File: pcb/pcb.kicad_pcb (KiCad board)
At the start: 2 copper layers, 7 parts, among them J1 Conn_01x16_Socket, J2 USB_C_Receptacle, U1 W65C02SxP, U2 W65C22SxP, U3 28C256, U4 28C256, U5 HM62256BLP

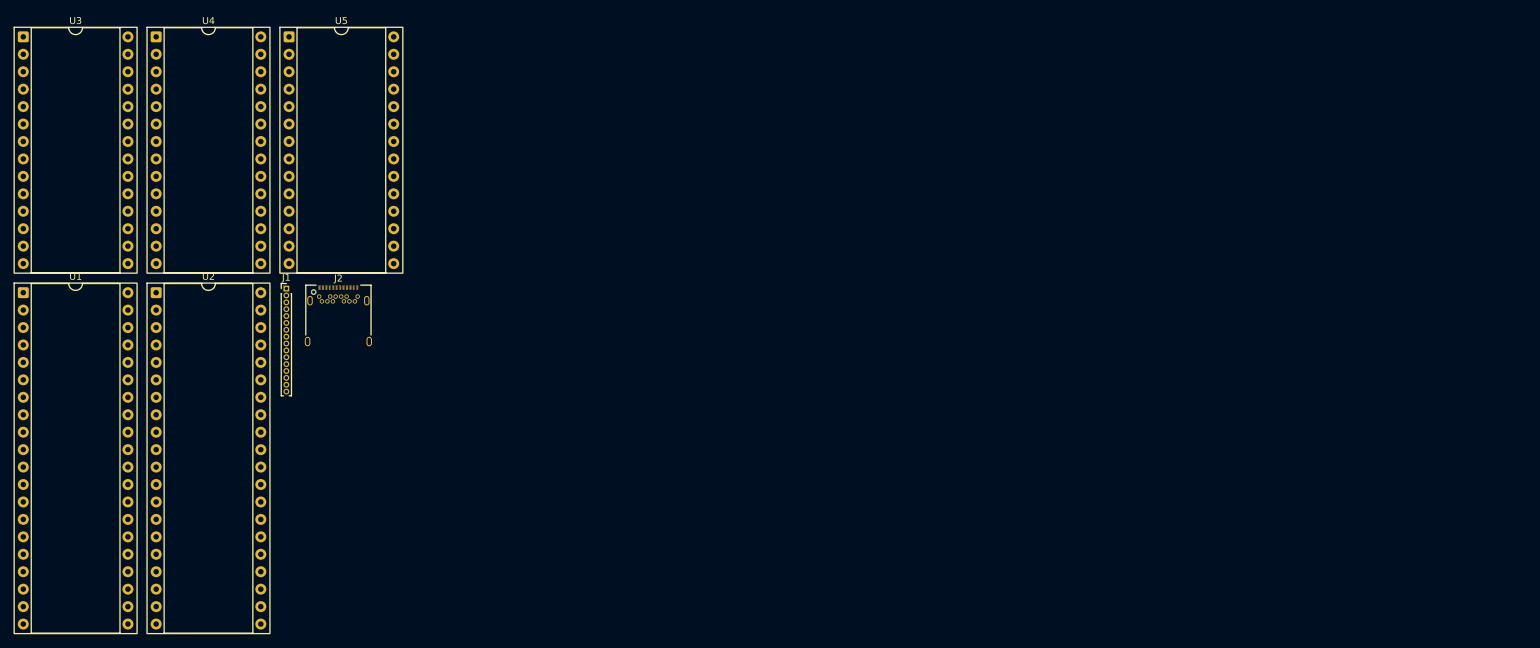
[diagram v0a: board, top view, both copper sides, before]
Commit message: lots of updates
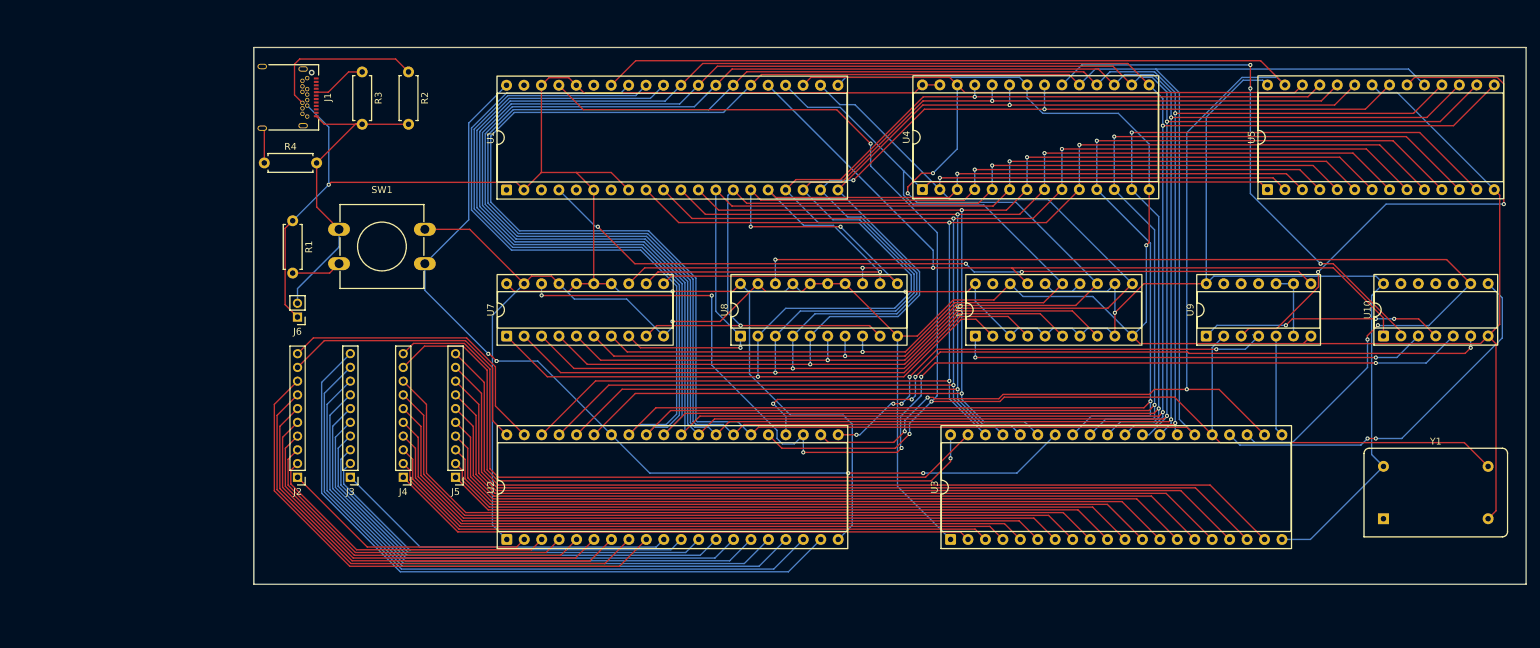
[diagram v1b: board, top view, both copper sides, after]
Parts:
- added J3: Conn_01x10_Pin, Connector_PinHeader_2.00mm:PinHeader_1x10_P2.00mm_Vertical, F.Cu at (76.5, 91.6)
- added J4: Conn_01x10_Pin, Connector_PinHeader_2.00mm:PinHeader_1x10_P2.00mm_Vertical, F.Cu at (84.2, 91.6)
- added J5: Conn_01x10_Pin, Connector_PinHeader_2.00mm:PinHeader_1x10_P2.00mm_Vertical, F.Cu at (91.9, 91.6)
- added J6: Conn_01x02_Pin, Connector_PinHeader_2.00mm:PinHeader_1x02_P2.00mm_Vertical, F.Cu at (68.8, 68.3)
- added R1: 220, Resistor_THT:R_Axial_DIN0207_L6.3mm_D2.5mm_P7.62mm_Horizontal, F.Cu at (68.1, 54.3)
- added R2: 5.11K, Resistor_THT:R_Axial_DIN0207_L6.3mm_D2.5mm_P7.62mm_Horizontal, F.Cu at (85.0, 32.6)
- added R3: 5.11K, Resistor_THT:R_Axial_DIN0207_L6.3mm_D2.5mm_P7.62mm_Horizontal, F.Cu at (78.3, 32.6)
- added R4: 1M, Resistor_THT:R_Axial_DIN0207_L6.3mm_D2.5mm_P7.62mm_Horizontal, F.Cu at (64.0, 45.9)
- added SW1: SW_Push, Button_Switch_THT:SW_PUSH-12mm, F.Cu at (74.9, 55.5)
- added U10: 74HC04, Package_DIP:DIP-14_W7.62mm_Socket, F.Cu at (227.0, 71.0)
- added U6: 74HC684, Package_DIP:DIP-20_W7.62mm_Socket, F.Cu at (167.6, 71.1)
- added U7: 74HC680, Package_DIP:DIP-20_W7.62mm_Socket, F.Cu at (99.3, 71.1)
- added U8: 74HC680, Package_DIP:DIP-20_W7.62mm_Socket, F.Cu at (133.3, 71.1)
- added U9: 74HC00, Package_DIP:DIP-14_W7.62mm_Socket, F.Cu at (201.2, 71.1)
- added Y1: MCO-1510A, Oscillator:Oscillator_DIP-14, F.Cu at (227.0, 97.7)
- J1: value Conn_01x16_Socket -> USB_C_Receptacle; footprint Connector_PinHeader_1.00mm:PinHeader_1x16_P1.00mm_Vertical -> Connector_USB:USB_C_Receptacle_Amphenol_12401548E4-2A
- J2: value USB_C_Receptacle -> Conn_01x10_Pin; footprint Connector_USB:USB_C_Receptacle_Amphenol_12401548E4-2A -> Connector_PinHeader_2.00mm:PinHeader_1x10_P2.00mm_Vertical
- U3: value 28C256 -> W65C22SxP; footprint Package_DIP:DIP-28_W15.24mm_Socket -> Package_DIP:DIP-40_W15.24mm_Socket
- moved U3 153.6 mm to (163.9, 100.7), turned to 90 degrees
- moved U5 144.2 mm to (210.1, 49.7), turned to 90 degrees
- moved U4 113.8 mm to (159.8, 49.7), turned to 90 degrees
- moved U1 71.9 mm to (99.3, 49.8), turned to 90 degrees
- moved U2 62.4 mm to (99.3, 100.7), turned to 90 degrees
- moved J1 27.9 mm to (66.5, 36.3), turned to -90 degrees
- moved J2 23.4 mm to (68.8, 91.6), turned to 180 degrees
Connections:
- U1 pad 2: unconnected-(U1-RDY-Pad2) -> +5V
- U1 pad 21: unconnected-(U1-VSS-Pad21) -> GND
- U1 pad 34: unconnected-(U1-R/~{W}-Pad34) -> R/~{W}
- U1 pad 36: unconnected-(U1-BE-Pad36) -> +5V
- U1 pad 37: unconnected-(U1-ϕ0-Pad37) -> CLK
- U1 pad 38: unconnected-(U1-~{SO}-Pad38) -> +5V
- U1 pad 4: unconnected-(U1-~{IRQ}-Pad4) -> Net-(U1-~{IRQ})
- U1 pad 40: unconnected-(U1-~{RES}-Pad40) -> ~{RES}
- U1 pad 6: unconnected-(U1-~{NMI}-Pad6) -> +5V
- U1 pad 8: unconnected-(U1-VDD-Pad8) -> +5V
- U2 pad 1: unconnected-(U2-VSS-Pad1) -> GND
- U2 pad 10: unconnected-(U2-PB0-Pad10) -> Net-(J3-Pin_1)
- U2 pad 11: unconnected-(U2-PB1-Pad11) -> Net-(J3-Pin_2)
- U2 pad 12: unconnected-(U2-PB2-Pad12) -> Net-(J3-Pin_3)
- U2 pad 13: unconnected-(U2-PB3-Pad13) -> Net-(J3-Pin_4)
- U2 pad 14: unconnected-(U2-PB4-Pad14) -> Net-(J3-Pin_5)
- U2 pad 15: unconnected-(U2-PB5-Pad15) -> Net-(J3-Pin_6)
- U2 pad 16: unconnected-(U2-PB6-Pad16) -> Net-(J3-Pin_7)
- U2 pad 17: unconnected-(U2-PB7-Pad17) -> Net-(J3-Pin_8)
- U2 pad 18: unconnected-(U2-CB1-Pad18) -> Net-(J3-Pin_9)
- U2 pad 19: unconnected-(U2-CB2-Pad19) -> Net-(J3-Pin_10)
- U2 pad 2: unconnected-(U2-PA0-Pad2) -> Net-(J2-Pin_1)
- U2 pad 20: unconnected-(U2-VCC-Pad20) -> +5V
- U2 pad 21: unconnected-(U2-~{IRQ}-Pad21) -> ~{IRQ} 1
- U2 pad 22: unconnected-(U2-R/~{W}-Pad22) -> R/~{W}
- U2 pad 23: unconnected-(U2-~{CS2}-Pad23) -> Net-(U2-~{CS2})
- U2 pad 24: unconnected-(U2-CS1-Pad24) -> Net-(U2-CS1)
- U2 pad 25: unconnected-(U2-ϕ2-Pad25) -> CLK
- U2 pad 3: unconnected-(U2-PA1-Pad3) -> Net-(J2-Pin_2)
- U2 pad 34: unconnected-(U2-~{RES}-Pad34) -> ~{RES}
- U2 pad 35: unconnected-(U2-RS3-Pad35) -> /A3
- U2 pad 36: unconnected-(U2-RS2-Pad36) -> /A2
- U2 pad 37: unconnected-(U2-RS1-Pad37) -> /A1
- U2 pad 38: unconnected-(U2-RS0-Pad38) -> /A0
- U2 pad 39: unconnected-(U2-CA2-Pad39) -> Net-(J2-Pin_10)
- U2 pad 4: unconnected-(U2-PA2-Pad4) -> Net-(J2-Pin_3)
- U2 pad 40: unconnected-(U2-CA1-Pad40) -> Net-(J2-Pin_9)
- U2 pad 5: unconnected-(U2-PA3-Pad5) -> Net-(J2-Pin_4)
- U2 pad 6: unconnected-(U2-PA4-Pad6) -> Net-(J2-Pin_5)
- U2 pad 7: unconnected-(U2-PA5-Pad7) -> Net-(J2-Pin_6)
- U2 pad 8: unconnected-(U2-PA6-Pad8) -> Net-(J2-Pin_7)
- U2 pad 9: unconnected-(U2-PA7-Pad9) -> Net-(J2-Pin_8)
- U3 pad 1: /A14 -> GND
- U3 pad 10: /A0 -> Net-(J5-Pin_1)
- U3 pad 11: /D0 -> Net-(J5-Pin_2)
- U3 pad 12: /D1 -> Net-(J5-Pin_3)
- U3 pad 13: /D2 -> Net-(J5-Pin_4)
- U3 pad 14: unconnected-(U3-GND-Pad14) -> Net-(J5-Pin_5)
- U3 pad 15: /D3 -> Net-(J5-Pin_6)
- U3 pad 16: /D4 -> Net-(J5-Pin_7)
- U3 pad 17: /D5 -> Net-(J5-Pin_8)
- U3 pad 18: /D6 -> Net-(J5-Pin_9)
- U3 pad 19: /D7 -> Net-(J5-Pin_10)
- U3 pad 2: /A12 -> Net-(J4-Pin_1)
- U3 pad 20: unconnected-(U3-~{CS}-Pad20) -> +5V
- U3 pad 21: /A10 -> ~{IRQ} 2
- U3 pad 22: unconnected-(U3-~{OE}-Pad22) -> R/~{W}
- U3 pad 23: /A11 -> Net-(U3-~{CS2})
- U3 pad 24: /A9 -> Net-(U3-CS1)
- U3 pad 25: /A8 -> CLK
- U3 pad 26: /A13 -> /D7
- U3 pad 27: unconnected-(U3-~{WE}-Pad27) -> /D6
- U3 pad 28: unconnected-(U3-VCC-Pad28) -> /D5
- U3 pad 3: /A7 -> Net-(J4-Pin_2)
- U3 pad 4: /A6 -> Net-(J4-Pin_3)
- U3 pad 5: /A5 -> Net-(J4-Pin_4)
- U3 pad 6: /A4 -> Net-(J4-Pin_5)
- U3 pad 7: /A3 -> Net-(J4-Pin_6)
- U3 pad 8: /A2 -> Net-(J4-Pin_7)
- U3 pad 9: /A1 -> Net-(J4-Pin_8)
- U4 pad 14: unconnected-(U4-GND-Pad14) -> GND
- U4 pad 20: unconnected-(U4-~{CS}-Pad20) -> Net-(U4-~{CS})
- U4 pad 22: unconnected-(U4-~{OE}-Pad22) -> GND
- U4 pad 27: unconnected-(U4-~{WE}-Pad27) -> +5V
- U4 pad 28: unconnected-(U4-VCC-Pad28) -> +5V
- U5 pad 14: unconnected-(U5-GND-Pad14) -> GND
- U5 pad 20: unconnected-(U5-~{CS}-Pad20) -> Net-(U5-~{CS})
- U5 pad 22: unconnected-(U5-~{OE}-Pad22) -> GND
- U5 pad 27: unconnected-(U5-~{WE}-Pad27) -> R/~{W}
- U5 pad 28: unconnected-(U5-VCC-Pad28) -> +5V
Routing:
- net +5V: track 0.00 -> 463.9 mm, vias 0 -> 4
- net GND: track 0.00 -> 452.8 mm, vias 0 -> 2
- net /D3: track 0.00 -> 348.6 mm, vias 0 -> 2
- net /D4: track 0.00 -> 342.8 mm, vias 0 -> 2
- net /D5: track 0.00 -> 338.0 mm, vias 0 -> 2
- net /D7: track 0.00 -> 337.0 mm
- net /D6: track 0.00 -> 334.1 mm, vias 0 -> 2
- net /D0: track 0.00 -> 285.7 mm, vias 0 -> 2
- net /D1: track 0.00 -> 281.7 mm, vias 0 -> 2
- net /D2: track 0.00 -> 277.7 mm, vias 0 -> 2
- net R/~{W}: track 0.00 -> 228.6 mm, vias 0 -> 3
- net /A10: track 0.00 -> 222.6 mm, vias 0 -> 3
- net /A0: track 0.00 -> 222.2 mm, vias 0 -> 3
- net /A8: track 0.00 -> 220.4 mm, vias 0 -> 2
- net CLK: track 0.00 -> 219.7 mm, vias 0 -> 3
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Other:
- board outline added: 185.3 x 78.2 mm
